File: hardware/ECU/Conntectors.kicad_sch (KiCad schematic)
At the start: 1 part

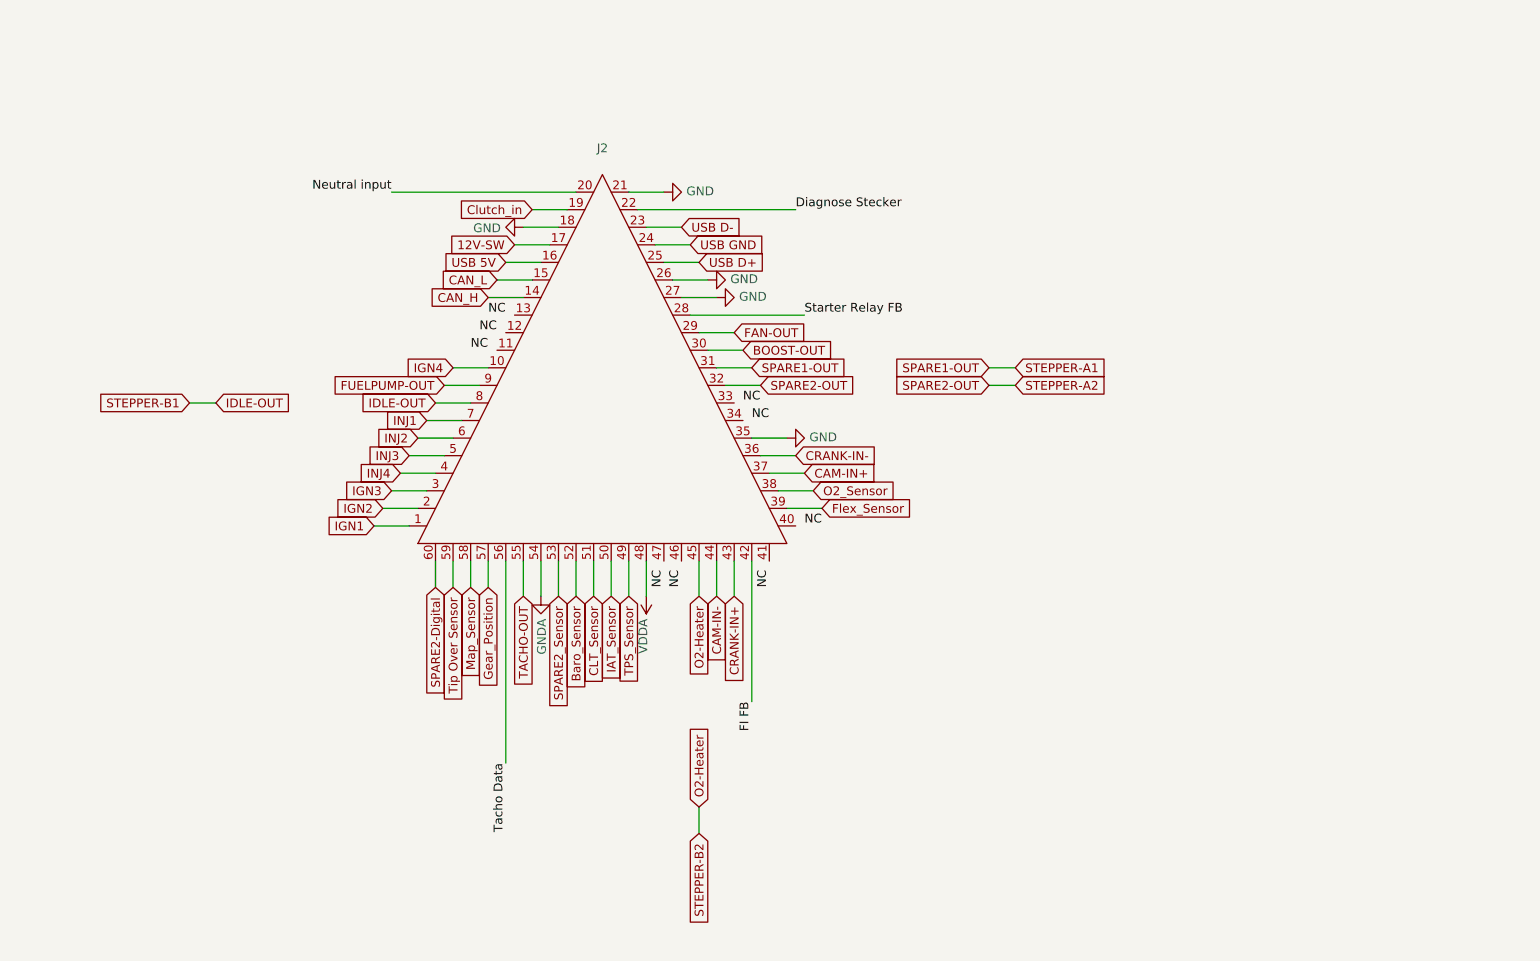
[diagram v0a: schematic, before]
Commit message: Update ECU-Hardware, Dokumente und Explosionszeichnungen
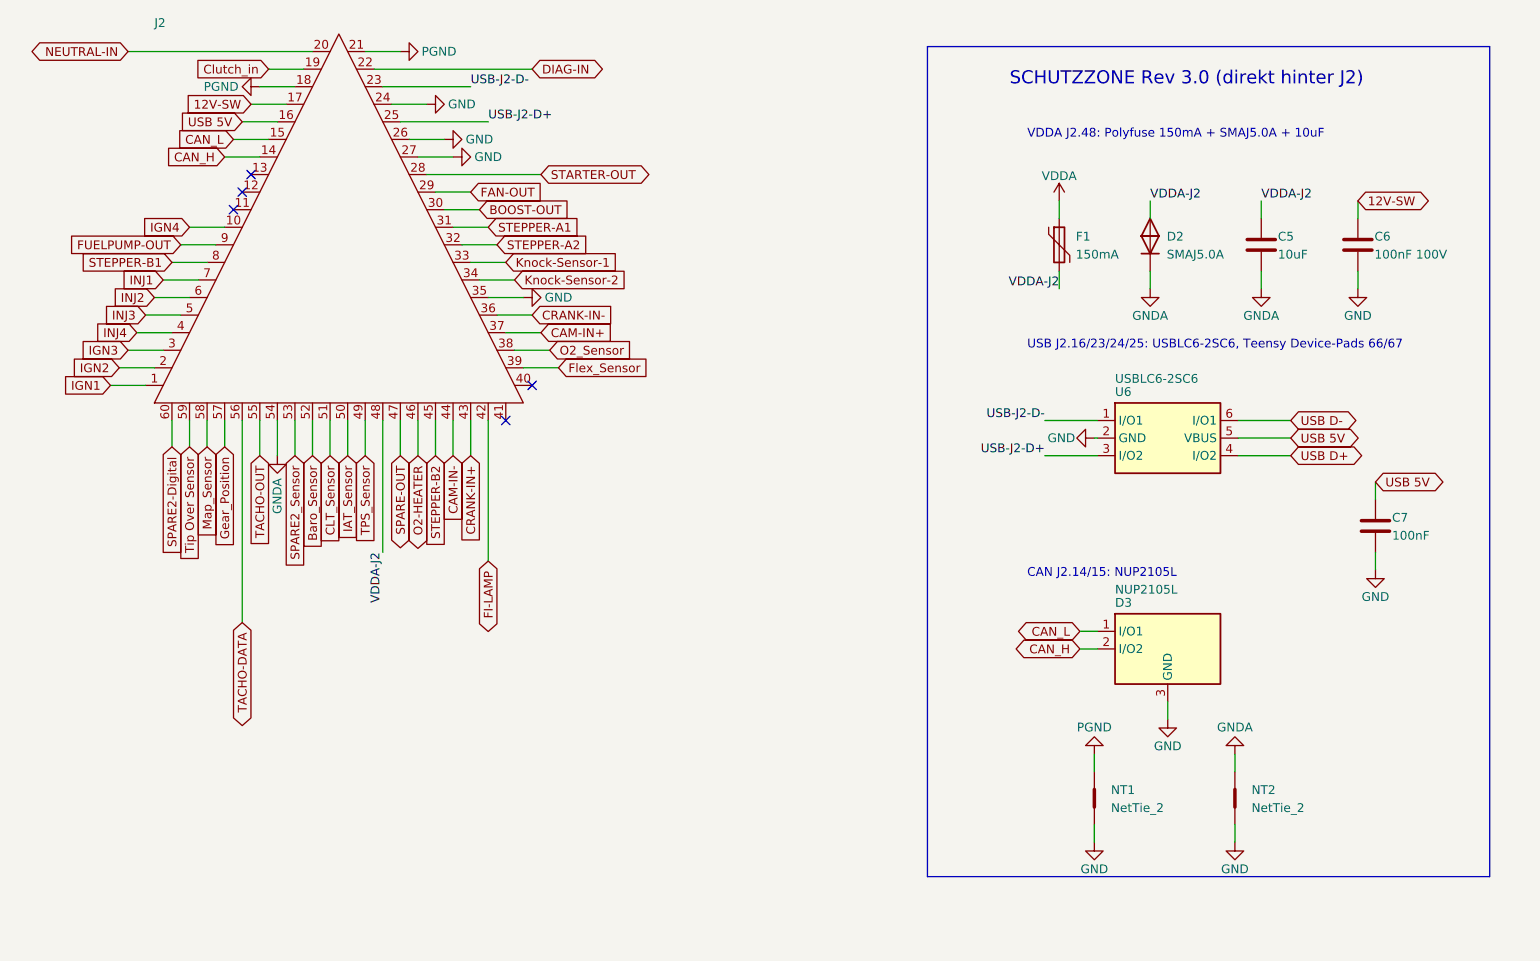
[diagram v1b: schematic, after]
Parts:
- added C5: 10uF, Capacitor_SMD:C_1206_3216Metric, symbol Device:C
- added C6: 100nF 100V, Capacitor_SMD:C_1206_3216Metric, symbol Device:C
- added C7: 100nF, Capacitor_SMD:C_0805_2012Metric, symbol Device:C
- added D2: SMAJ5.0A, Diode_SMD:D_SMA, symbol Device:D_TVS
- added D3: NUP2105L, Package_TO_SOT_SMD:SOT-23, symbol Rev3:NUP2105L
- added F1: 150mA, Fuse:Fuse_1812_4532Metric, symbol Device:Polyfuse
- added NT1, NT2: NetTie_2, NetTie:NetTie-2_SMD_Pad0.5mm, symbol Device:NetTie_2
- added U6: USBLC6-2SC6, Package_TO_SOT_SMD:SOT-23-6, symbol Rev3:USBLC6-2SC6
- J2: value ~ -> (none); BOM Comments (none) -> Gegenstueck/Kontakte separat beschaffen (SUPERSEAL 1.0 60-p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; Digikey Part Number (none) -> A122211-ND; Manufacturer_Name (none) -> TE Connectivity; Manufacturer_Part_Number (none) -> 6437288-3; Supplier (none) -> DigiKey; now left out of the parts list
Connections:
- net USB GND is gone; now on net GND: J2.24
- net 12V-SW: now also C6.1
- net CAN_H: now also D3.2 (I/O2)
- net CAN_L: now also D3.1 (I/O1)
- net GND: now also C6.2, C7.2, D3.3 (GND), NT1.2, NT2.2, U6.2 (GND); no longer J2.18, J2.21
- net GNDA: now also C5.2, D2.2, NT2.1
- net USB 5V: now also C7.1, U6.5 (VBUS)
- net USB D+: now also U6.4 (I/O2); no longer J2.25
- net USB D-: now also U6.6 (I/O1); no longer J2.23
- net VDDA: now also F1.1; no longer J2.48
- net Knock-Sensor-1: now reaches J2.33
- net Knock-Sensor-2: now reaches J2.34
- net O2-HEATER: now reaches J2.46
- net SPARE-OUT: now reaches J2.47
- net Diagnose Stecker renamed DIAG-IN
- net FI FB renamed FI-LAMP
- net IDLE-OUT renamed STEPPER-B1
- net Neutral input renamed NEUTRAL-IN
- net O2-Heater renamed STEPPER-B2
- net SPARE1-OUT renamed STEPPER-A1
- net SPARE2-OUT renamed STEPPER-A2
- net Starter Relay FB renamed STARTER-OUT
- net Tacho Data renamed TACHO-DATA
- new net PGND: J2.18, J2.21, NT1.1
- new net USB-J2-D+: J2.25, U6.3 (I/O2)
- new net USB-J2-D-: J2.23, U6.1 (I/O1)
- new net VDDA-J2: C5.1, D2.1, F1.2, J2.48
- no-connect marks 0 -> 5
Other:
- note added: "CAN J2.14/15: NUP2105L"
- note added: "SCHUTZZONE Rev 3.0 (direkt hinter J2)"
- note added: "USB J2.16/23/24/25: USBLC6-2SC6, Teensy Device-Pads 66/67"
- note added: "VDDA J2.48: Polyfuse 150mA + SMAJ5.0A + 10uF"
- title: (none) -> Connectors
- moved on the sheet: J2
